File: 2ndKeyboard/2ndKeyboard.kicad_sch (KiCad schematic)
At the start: 197 parts, among them J1 AVR-ISP-6, K1 ESC, K10 F9, K11 F10, K12 F11, K13 F12, K14 Imp_Ecran, K15 Defilement, K16 Pause, K17 /, K18 1, K19 2, K2 F1, K20 3, K21 4, K22 5, K23 6, K24 7, K25 8, K26 9, K27 0, K28 -, K29 =, K3 F2, K30 KEYSW, K31 Ins, K32 Debut, K33 Next, K34 TAB, K35 Q, K36 W, K37 E, K38 R, K39 T, K4 F3, K40 Y, K41 U, K42 I, K43 O, K44 P, K45 ^, K46 Ç, K47 À, K48 Suppr, K49 FIN, K5 F4, K50 Previous, K51 CAPS LOCK, K52 A, K53 S, K54 D, K55 F, K56 G, K57 H, K58 J, K59 K, K6 F5, K60 L, K61 ;, K62 È, K63 ENTER, K64 MAJ G., K65 Z, K66 X, K67 C, K68 V, K69 B, K7 F6, K70 N, K71 M, K72 ,, K73 ., K74 É, K75 MAJ D., K76 UP Arrow, K77 CTRL G., K78 WINDOWS, K79 ALT G., K8 F7, K80 BARRE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

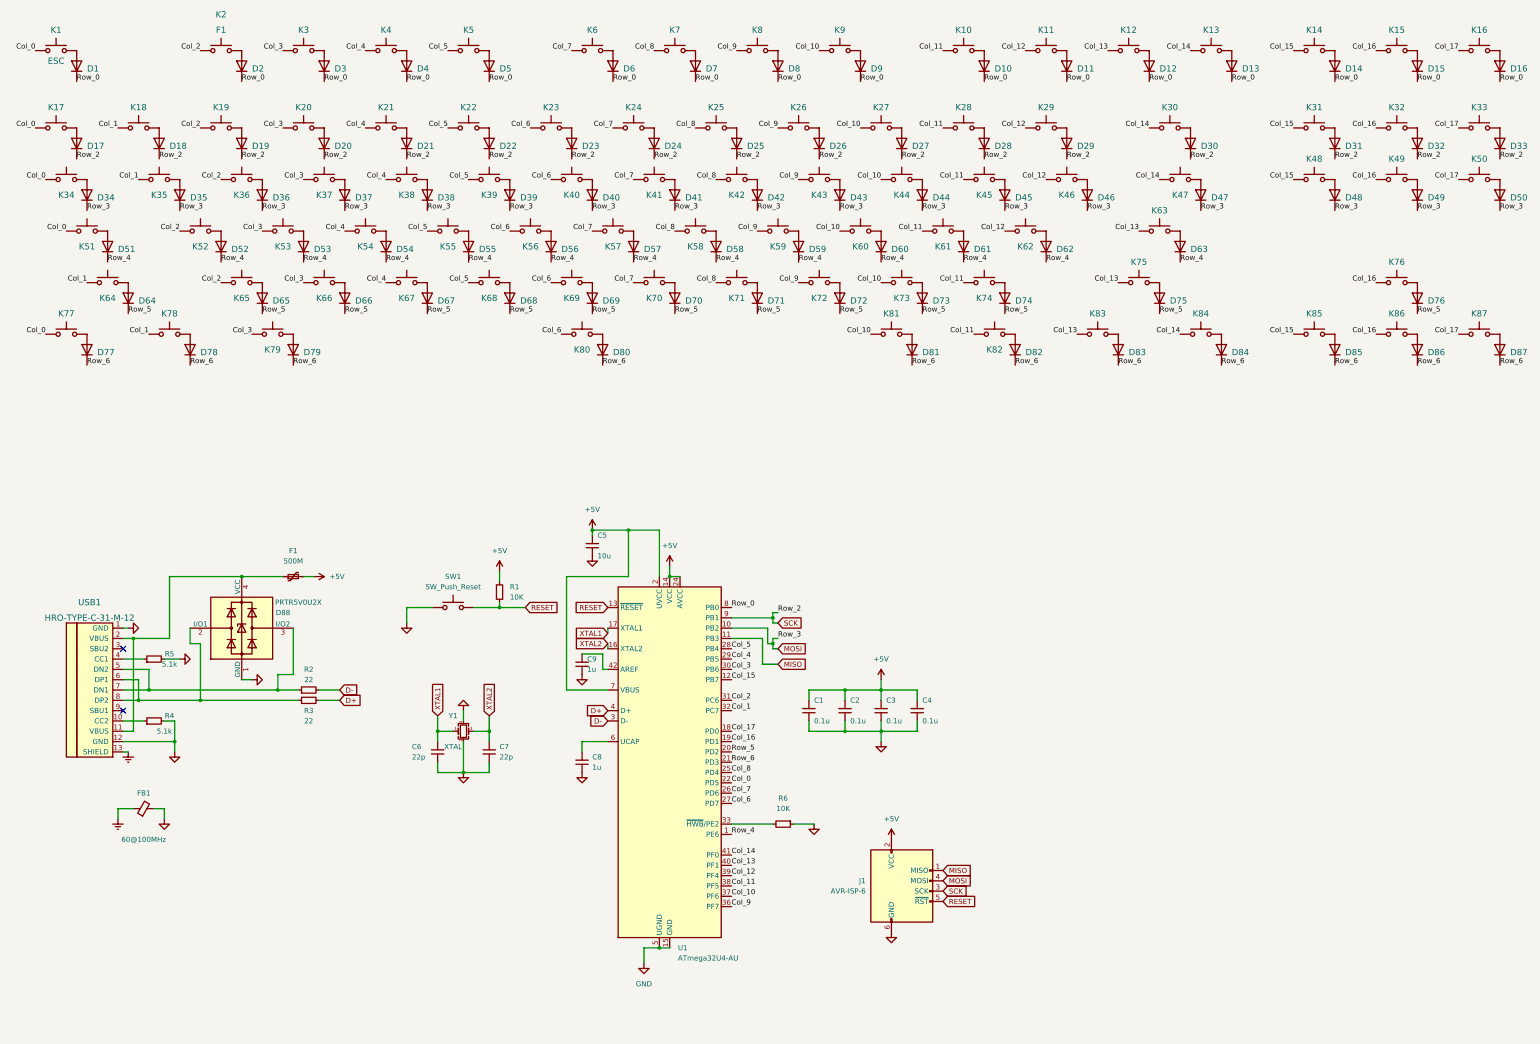
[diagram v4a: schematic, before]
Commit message: PCB & Schematic 20230108a
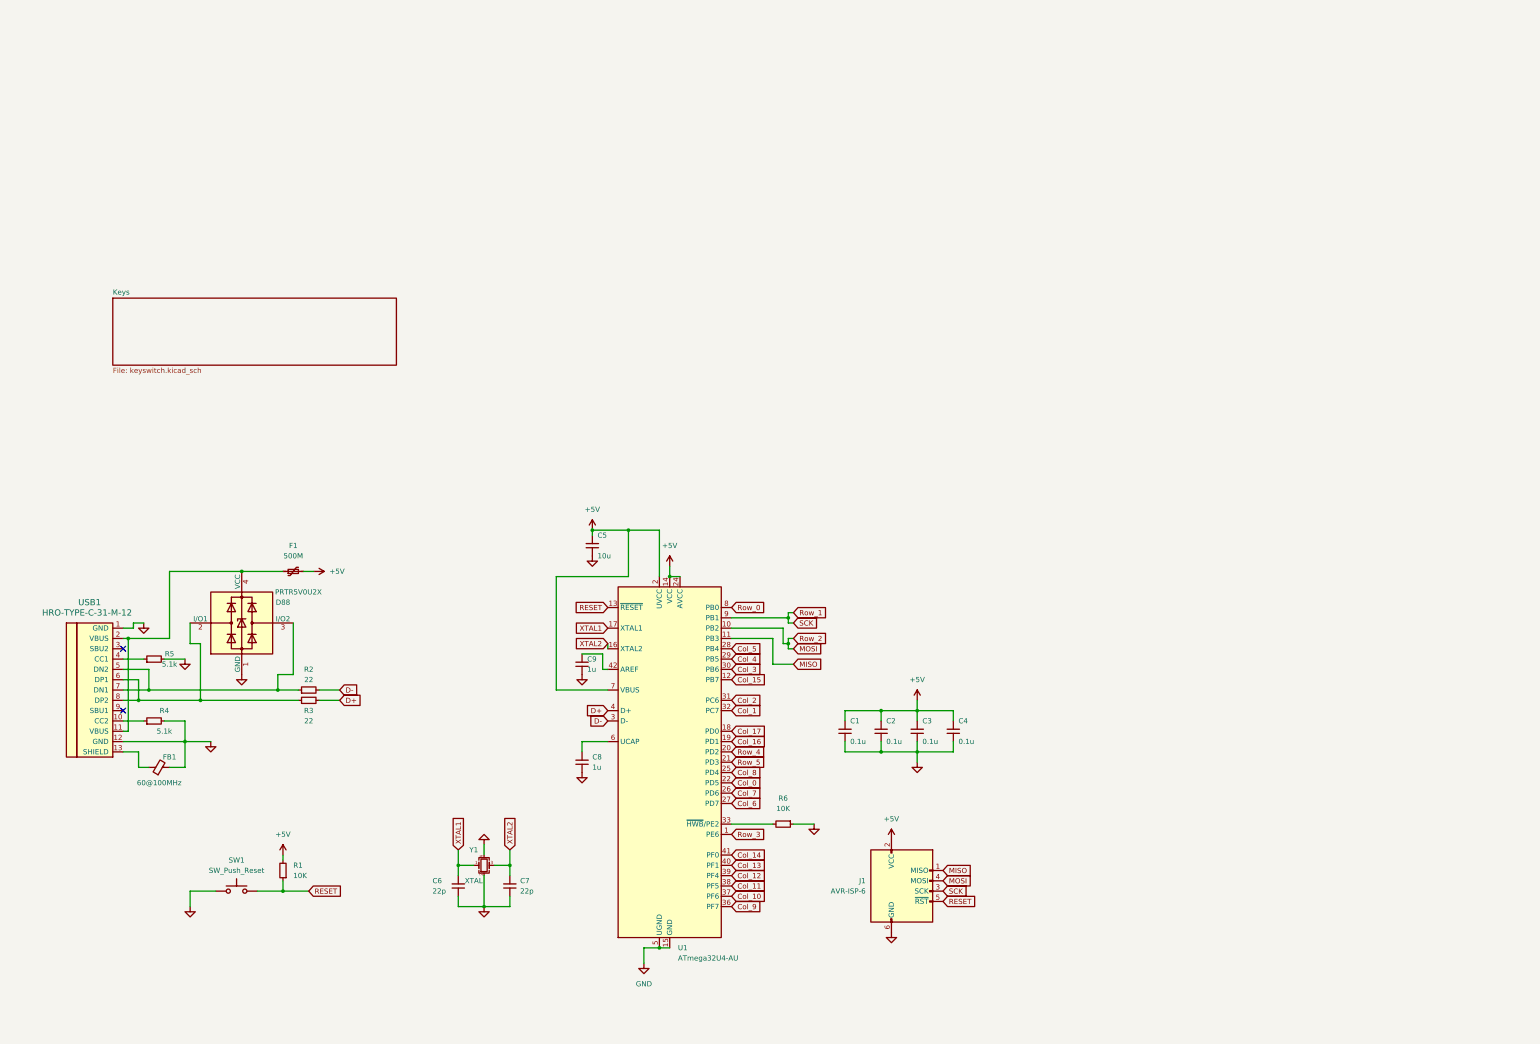
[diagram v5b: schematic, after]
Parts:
- removed D1, D10, D11, D12, D13, D14, D15, D16, D17, D18, D19, D2, D20, D21, D22, D23, D24, D25, D26, D27, D28, D29, D3, D30, D31, D32, D33, D34, D35, D36, D37, D38, D39, D4, D40, D41, D42, D43, D44, D45, D46, D47, D48, D49, D5, D50, D51, D52, D53, D54, D55, D56, D57, D58, D59, D6, D60, D61, D62, D63, D64, D65, D66, D67, D68, D69, D7, D70, D71, D72, D73, D74, D75, D76, D77, D78, D79, D8, D80, D81, D82, D83, D84, D85, D86, D87, D9: D, Diode_SMD:D_SOD-123, symbol Device:D
- removed K1: ESC, Button_Switch_Keyboard:SW_Cherry_MX_1.00u_PCB, symbol Switch:SW_Push
- removed K10: F9, Button_Switch_Keyboard:SW_Cherry_MX_1.00u_PCB, symbol Switch:SW_Push
- removed K11: F10, Button_Switch_Keyboard:SW_Cherry_MX_1.00u_PCB, symbol Switch:SW_Push
- removed K12: F11, Button_Switch_Keyboard:SW_Cherry_MX_1.00u_PCB, symbol Switch:SW_Push
- removed K13: F12, Button_Switch_Keyboard:SW_Cherry_MX_1.00u_PCB, symbol Switch:SW_Push
- removed K14: Imp_Ecran, Button_Switch_Keyboard:SW_Cherry_MX_1.00u_PCB, symbol Switch:SW_Push
- removed K15: Defilement, Button_Switch_Keyboard:SW_Cherry_MX_1.00u_PCB, symbol Switch:SW_Push
- removed K16: Pause, Button_Switch_Keyboard:SW_Cherry_MX_1.00u_PCB, symbol Switch:SW_Push
- removed K17: /, Button_Switch_Keyboard:SW_Cherry_MX_1.00u_PCB, symbol Switch:SW_Push
- removed K18: 1, Button_Switch_Keyboard:SW_Cherry_MX_1.00u_PCB, symbol Switch:SW_Push
- removed K19: 2, Button_Switch_Keyboard:SW_Cherry_MX_1.00u_PCB, symbol Switch:SW_Push
- removed K2: F1, Button_Switch_Keyboard:SW_Cherry_MX_1.00u_PCB, symbol Switch:SW_Push
- removed K20: 3, Button_Switch_Keyboard:SW_Cherry_MX_1.00u_PCB, symbol Switch:SW_Push
- removed K21: 4, Button_Switch_Keyboard:SW_Cherry_MX_1.00u_PCB, symbol Switch:SW_Push
- removed K22: 5, Button_Switch_Keyboard:SW_Cherry_MX_1.00u_PCB, symbol Switch:SW_Push
- removed K23: 6, Button_Switch_Keyboard:SW_Cherry_MX_1.00u_PCB, symbol Switch:SW_Push
- removed K24: 7, Button_Switch_Keyboard:SW_Cherry_MX_1.00u_PCB, symbol Switch:SW_Push
- removed K25: 8, Button_Switch_Keyboard:SW_Cherry_MX_1.00u_PCB, symbol Switch:SW_Push
- removed K26: 9, Button_Switch_Keyboard:SW_Cherry_MX_1.00u_PCB, symbol Switch:SW_Push
- removed K27: 0, Button_Switch_Keyboard:SW_Cherry_MX_1.00u_PCB, symbol Switch:SW_Push
- removed K28: -, Button_Switch_Keyboard:SW_Cherry_MX_1.00u_PCB, symbol Switch:SW_Push
- removed K29: =, Button_Switch_Keyboard:SW_Cherry_MX_1.00u_PCB, symbol Switch:SW_Push
- removed K3: F2, Button_Switch_Keyboard:SW_Cherry_MX_1.00u_PCB, symbol Switch:SW_Push
- removed K30: KEYSW, Button_Switch_Keyboard:SW_Cherry_MX_2.00u_PCB, symbol Switch:SW_Push
- removed K31: Ins, Button_Switch_Keyboard:SW_Cherry_MX_1.00u_PCB, symbol Switch:SW_Push
- removed K32: Debut, Button_Switch_Keyboard:SW_Cherry_MX_1.00u_PCB, symbol Switch:SW_Push
- removed K33: Next, Button_Switch_Keyboard:SW_Cherry_MX_1.00u_PCB, symbol Switch:SW_Push
- removed K34: TAB, Button_Switch_Keyboard:SW_Cherry_MX_1.25u_PCB, symbol Switch:SW_Push
- removed K35: Q, Button_Switch_Keyboard:SW_Cherry_MX_1.00u_PCB, symbol Switch:SW_Push
- removed K36: W, Button_Switch_Keyboard:SW_Cherry_MX_1.00u_PCB, symbol Switch:SW_Push
- removed K37: E, Button_Switch_Keyboard:SW_Cherry_MX_1.00u_PCB, symbol Switch:SW_Push
- removed K38: R, Button_Switch_Keyboard:SW_Cherry_MX_1.00u_PCB, symbol Switch:SW_Push
- removed K39: T, Button_Switch_Keyboard:SW_Cherry_MX_1.00u_PCB, symbol Switch:SW_Push
- removed K4: F3, Button_Switch_Keyboard:SW_Cherry_MX_1.00u_PCB, symbol Switch:SW_Push
- removed K40: Y, Button_Switch_Keyboard:SW_Cherry_MX_1.00u_PCB, symbol Switch:SW_Push
- removed K41: U, Button_Switch_Keyboard:SW_Cherry_MX_1.00u_PCB, symbol Switch:SW_Push
- removed K42: I, Button_Switch_Keyboard:SW_Cherry_MX_1.00u_PCB, symbol Switch:SW_Push
- removed K43: O, Button_Switch_Keyboard:SW_Cherry_MX_1.00u_PCB, symbol Switch:SW_Push
- removed K44: P, Button_Switch_Keyboard:SW_Cherry_MX_1.00u_PCB, symbol Switch:SW_Push
- removed K45: ^, Button_Switch_Keyboard:SW_Cherry_MX_1.00u_PCB, symbol Switch:SW_Push
- removed K46: Ç, Button_Switch_Keyboard:SW_Cherry_MX_1.00u_PCB, symbol Switch:SW_Push
- removed K47: À, Button_Switch_Keyboard:SW_Cherry_MX_1.75u_PCB, symbol Switch:SW_Push
- removed K48: Suppr, Button_Switch_Keyboard:SW_Cherry_MX_1.00u_PCB, symbol Switch:SW_Push
- removed K49: FIN, Button_Switch_Keyboard:SW_Cherry_MX_1.00u_PCB, symbol Switch:SW_Push
- removed K5: F4, Button_Switch_Keyboard:SW_Cherry_MX_1.00u_PCB, symbol Switch:SW_Push
- removed K50: Previous, Button_Switch_Keyboard:SW_Cherry_MX_1.00u_PCB, symbol Switch:SW_Push
- removed K51: CAPS LOCK, Button_Switch_Keyboard:SW_Cherry_MX_1.75u_PCB, symbol Switch:SW_Push
- removed K52: A, Button_Switch_Keyboard:SW_Cherry_MX_1.00u_PCB, symbol Switch:SW_Push
- removed K53: S, Button_Switch_Keyboard:SW_Cherry_MX_1.00u_PCB, symbol Switch:SW_Push
- removed K54: D, Button_Switch_Keyboard:SW_Cherry_MX_1.00u_PCB, symbol Switch:SW_Push
- removed K55: F, Button_Switch_Keyboard:SW_Cherry_MX_1.00u_PCB, symbol Switch:SW_Push
- removed K56: G, Button_Switch_Keyboard:SW_Cherry_MX_1.00u_PCB, symbol Switch:SW_Push
- removed K57: H, Button_Switch_Keyboard:SW_Cherry_MX_1.00u_PCB, symbol Switch:SW_Push
- removed K58: J, Button_Switch_Keyboard:SW_Cherry_MX_1.00u_PCB, symbol Switch:SW_Push
- removed K59: K, Button_Switch_Keyboard:SW_Cherry_MX_1.00u_PCB, symbol Switch:SW_Push
- removed K6: F5, Button_Switch_Keyboard:SW_Cherry_MX_1.00u_PCB, symbol Switch:SW_Push
- removed K60: L, Button_Switch_Keyboard:SW_Cherry_MX_1.00u_PCB, symbol Switch:SW_Push
- removed K61: ;, Button_Switch_Keyboard:SW_Cherry_MX_1.00u_PCB, symbol Switch:SW_Push
- removed K62: È, Button_Switch_Keyboard:SW_Cherry_MX_1.00u_PCB, symbol Switch:SW_Push
- removed K63: ENTER, Button_Switch_Keyboard:SW_Cherry_MX_2.25u_PCB, symbol Switch:SW_Push
- removed K64: MAJ G., Button_Switch_Keyboard:SW_Cherry_MX_2.25u_PCB, symbol Switch:SW_Push
- removed K65: Z, Button_Switch_Keyboard:SW_Cherry_MX_1.00u_PCB, symbol Switch:SW_Push
- removed K66: X, Button_Switch_Keyboard:SW_Cherry_MX_1.00u_PCB, symbol Switch:SW_Push
- removed K67: C, Button_Switch_Keyboard:SW_Cherry_MX_1.00u_PCB, symbol Switch:SW_Push
- removed K68: V, Button_Switch_Keyboard:SW_Cherry_MX_1.00u_PCB, symbol Switch:SW_Push
- removed K69: B, Button_Switch_Keyboard:SW_Cherry_MX_1.00u_PCB, symbol Switch:SW_Push
- removed K7: F6, Button_Switch_Keyboard:SW_Cherry_MX_1.00u_PCB, symbol Switch:SW_Push
- removed K70: N, Button_Switch_Keyboard:SW_Cherry_MX_1.00u_PCB, symbol Switch:SW_Push
- removed K71: M, Button_Switch_Keyboard:SW_Cherry_MX_1.00u_PCB, symbol Switch:SW_Push
- removed K72: ,, Button_Switch_Keyboard:SW_Cherry_MX_1.00u_PCB, symbol Switch:SW_Push
- removed K73: ., Button_Switch_Keyboard:SW_Cherry_MX_1.00u_PCB, symbol Switch:SW_Push
- removed K74: É, Button_Switch_Keyboard:SW_Cherry_MX_1.00u_PCB, symbol Switch:SW_Push
- removed K75: MAJ D., Button_Switch_Keyboard:SW_Cherry_MX_2.75u_PCB, symbol Switch:SW_Push
- removed K76: UP Arrow, Button_Switch_Keyboard:SW_Cherry_MX_1.00u_PCB, symbol Switch:SW_Push
- removed K77: CTRL G., Button_Switch_Keyboard:SW_Cherry_MX_1.25u_PCB, symbol Switch:SW_Push
- removed K78, K82: WINDOWS, Button_Switch_Keyboard:SW_Cherry_MX_1.25u_PCB, symbol Switch:SW_Push
- removed K79: ALT G., Button_Switch_Keyboard:SW_Cherry_MX_1.25u_PCB, symbol Switch:SW_Push
- removed K8: F7, Button_Switch_Keyboard:SW_Cherry_MX_1.00u_PCB, symbol Switch:SW_Push
- removed K80: BARRE, Button_Switch_Keyboard:SW_Cherry_MX_6.25u_PCB, symbol Switch:SW_Push
- removed K81: ALT D., Button_Switch_Keyboard:SW_Cherry_MX_1.25u_PCB, symbol Switch:SW_Push
- removed K83: MENU, Button_Switch_Keyboard:SW_Cherry_MX_1.25u_PCB, symbol Switch:SW_Push
- removed K84: CTRL D., Button_Switch_Keyboard:SW_Cherry_MX_1.25u_PCB, symbol Switch:SW_Push
- removed K85: LEFT Arrow, Button_Switch_Keyboard:SW_Cherry_MX_1.00u_PCB, symbol Switch:SW_Push
- removed K86: DOWN Arrow, Button_Switch_Keyboard:SW_Cherry_MX_1.00u_PCB, symbol Switch:SW_Push
- removed K87: RIGHT Arrow, Button_Switch_Keyboard:SW_Cherry_MX_1.00u_PCB, symbol Switch:SW_Push
- removed K9: F8, Button_Switch_Keyboard:SW_Cherry_MX_1.00u_PCB, symbol Switch:SW_Push
- D88: footprint random-keyboard-parts:SOT143B -> Package_TO_SOT_SMD:SOT-143
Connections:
- net Row_6 is gone; now on net Row_5: U1.21 (PD3)
- net Row_4: now also U1.20 (PD2); no longer U1.1 (PE6)
- net Row_5: no longer U1.20 (PD2)
- net Earth: no longer names the net of FB1.1, USB1.13 (SHIELD)
- net SCK renamed Row_1
- new net Row_3: U1.1 (PE6)
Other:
- added sheet Keys (keyswitch.kicad_sch)
- moved on the sheet: C1, C2, C3, C4, C6, C7, D88, F1, FB1, R1, SW1, Y1
